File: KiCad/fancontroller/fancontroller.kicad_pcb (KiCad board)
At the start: 2 copper layers, 25.7 x 36.8 mm, 14 parts, among them IC1 NE555DR, IC2 LM311DR, IC3 NE555DR

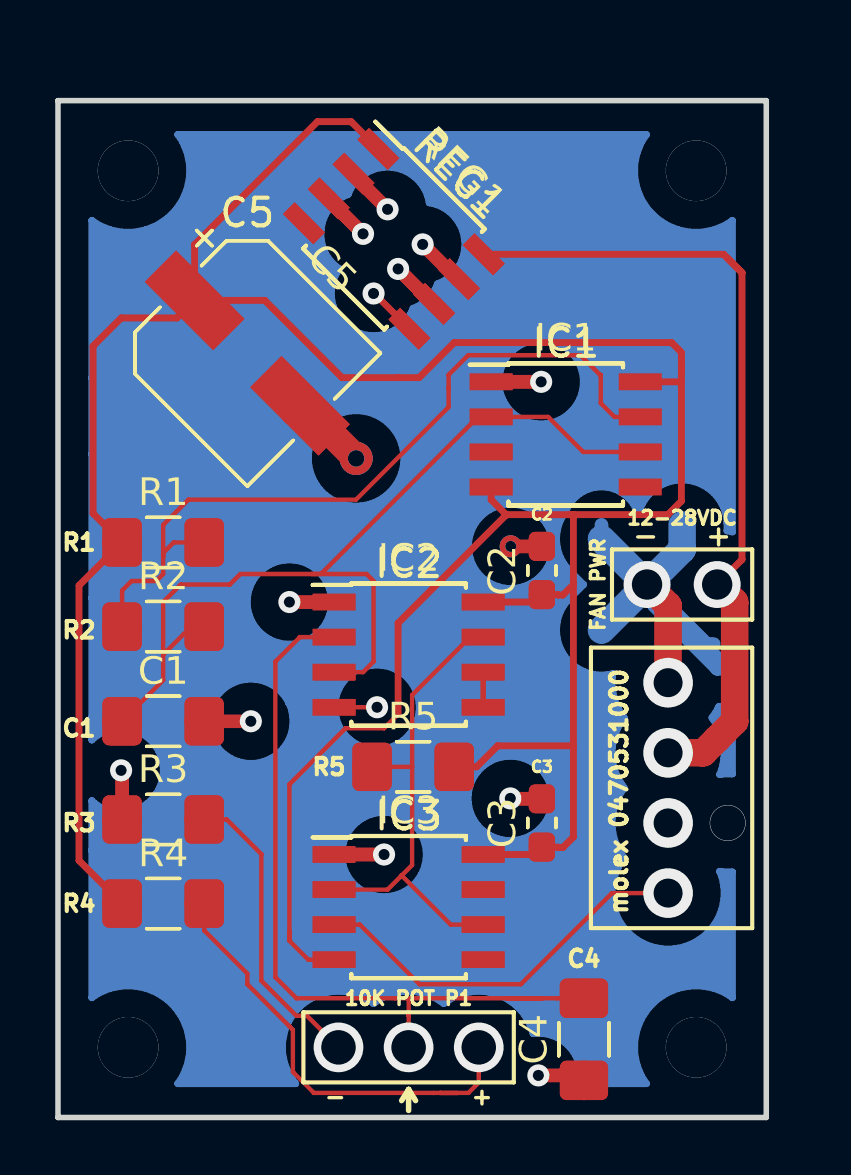
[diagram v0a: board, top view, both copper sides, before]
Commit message: feat: save PCB reconstruction checkpoint and detailed passdown
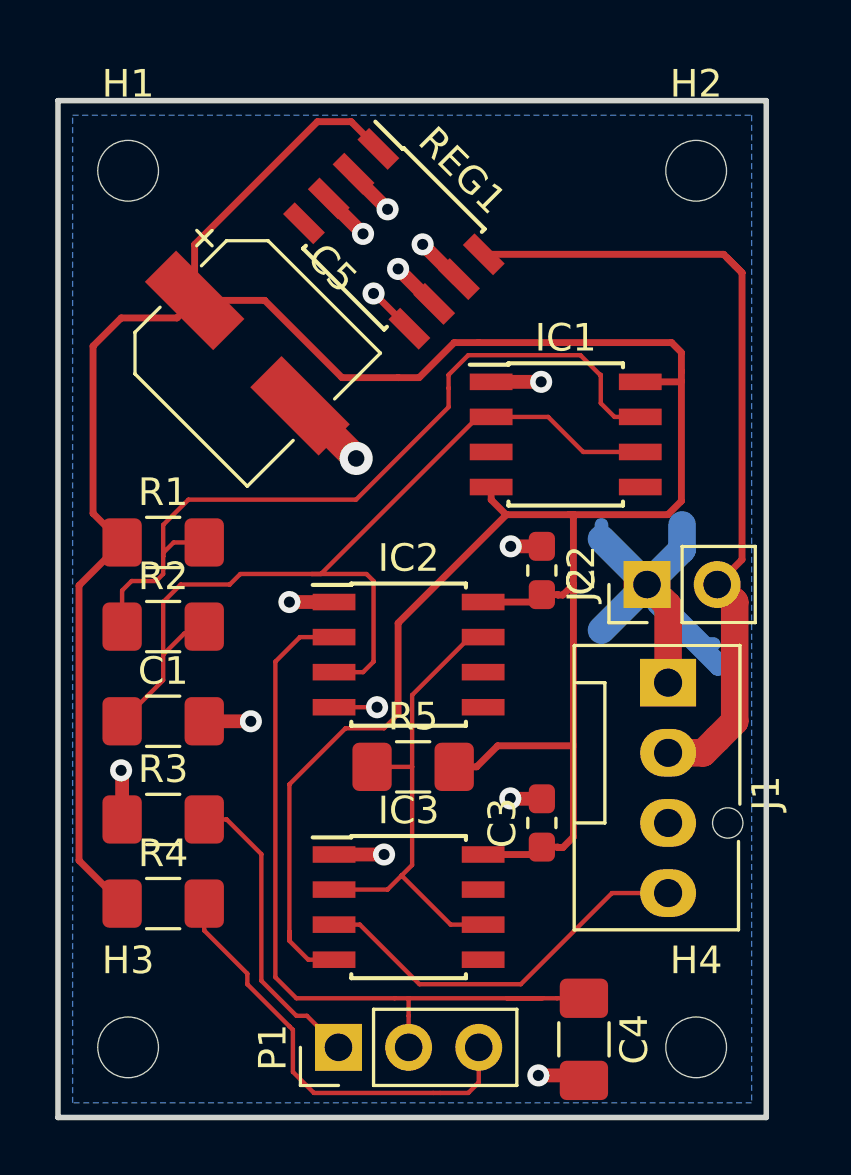
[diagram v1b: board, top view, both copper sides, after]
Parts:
- added H1: M2 mounting hole, MountingHole:MountingHole_2.2mm_M2, F.Cu at (80.0, 141.0)
- added H2: M2 mounting hole, MountingHole:MountingHole_2.2mm_M2, F.Cu at (100.6, 141.0)
- added H3: M2 mounting hole, MountingHole:MountingHole_2.2mm_M2, F.Cu at (80.0, 172.7)
- added H4: M2 mounting hole, MountingHole:MountingHole_2.2mm_M2, F.Cu at (100.6, 172.7)
- added J1: Fan 4-pin, Connector:FanPinHeader_1x04_P2.54mm_Vertical, F.Cu at (99.6, 159.5)
- added J2: Power input, Connector_PinHeader_2.54mm:PinHeader_1x02_P2.54mm_Vertical, F.Cu at (98.8, 156.0)
- added P1: 10k, Connector_PinHeader_2.54mm:PinHeader_1x03_P2.54mm_Vertical, F.Cu at (87.6, 172.7)
- C5: value 47uF 10V -> 47uF 35V
- REG1: value TS2938CS50 -> KF50BD-TR
- turned C4 to -90 degrees
- turned C2 to -90 degrees
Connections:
- C1 pad 1: (no net) -> RAMP
- C1 pad 2: (no net) -> GND
- C2 pad 1: (no net) -> GND
- C2 pad 2: (no net) -> +5V
- C3 pad 1: (no net) -> +5V
- C3 pad 2: (no net) -> GND
- C4 pad 1: (no net) -> DUTY_REF
- C4 pad 2: (no net) -> GND
- C5 pad 1: (no net) -> +5V
- C5 pad 2: (no net) -> GND
- IC1 pad 1: (no net) -> GND
- IC1 pad 2: (no net) -> RAMP
- IC1 pad 4: (no net) -> +5V
- IC1 pad 6: (no net) -> RAMP
- IC1 pad 7: (no net) -> DISCHARGE
- IC1 pad 8: (no net) -> +5V
- IC2 pad 1: (no net) -> GND
- IC2 pad 2: (no net) -> DUTY_REF
- IC2 pad 3: (no net) -> RAMP
- IC2 pad 4: (no net) -> GND
- IC2 pad 7: (no net) -> COMPARATOR
- IC2 pad 8: (no net) -> +5V
- IC3 pad 1: (no net) -> GND
- IC3 pad 2: (no net) -> COMPARATOR
- IC3 pad 3: (no net) -> PWM_OUT
- IC3 pad 4: (no net) -> +5V
- IC3 pad 6: (no net) -> COMPARATOR
- IC3 pad 8: (no net) -> +5V
- R1 pad 1: (no net) -> +5V
- R1 pad 2: (no net) -> DISCHARGE
- R2 pad 1: (no net) -> DISCHARGE
- R2 pad 2: (no net) -> RAMP
- R3 pad 1: (no net) -> GND
- R3 pad 2: (no net) -> POT_LOW
- R4 pad 1: (no net) -> +5V
- R4 pad 2: (no net) -> POT_HIGH
- R5 pad 1: (no net) -> COMPARATOR
- R5 pad 2: (no net) -> +5V
- REG1 pad 1: (no net) -> +5V
- REG1 pad 2: (no net) -> GND
- REG1 pad 3: (no net) -> GND
- REG1 pad 5: (no net) -> GND
- REG1 pad 6: (no net) -> GND
- REG1 pad 7: (no net) -> GND
- REG1 pad 8: (no net) -> +12V
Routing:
- net (no net): track 747.3 -> 0.00 mm, vias 29 -> 0
- net +5V: track 0.00 -> 118.8 mm
- net GND: track 0.00 -> 47.4 mm, vias 0 -> 15
- net RAMP: track 0.00 -> 34.3 mm
- net +12V: track 0.00 -> 30.2 mm
- net DISCHARGE: track 0.00 -> 28.6 mm
- net DUTY_REF: track 0.00 -> 28.5 mm
- net COMPARATOR: track 0.00 -> 17.9 mm
- net POT_HIGH: track 0.00 -> 15.9 mm
- net PWM_OUT: track 0.00 -> 14.4 mm
- net POT_LOW: track 0.00 -> 11.0 mm
- added copper zone on B.Cu, net GND
